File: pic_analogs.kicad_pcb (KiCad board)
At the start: 2 copper layers, 99.1 x 98.4 mm, 226 parts, among them J1 VFWD, J10 USB_B_Mini, J11 term_, J12 term_, J13 term_, J14 term_, J15 term_, J16 term_, J17 term_, J18 term_, J19 term_, J2 IN_RF, J20 term_, J21 term_, J22 term_, J23 term_, J24 term_, J25 term_, J26 term_, J27 term_, J28 term_, J29 term_, J3 OUT_RF, J30 term_, J31 term_, J32 ICD, J33 Micro_SD_Card, J34 Raspberry_Pi_zero_2w, J35 USB_A, J36 OledSpiST1306, J37 OledSpiST7789, J4 VREV, J42 OledSpiST1306, J43 tp_ft232_, J44 tp_ft232_, J45 tp_ft232_, J46 tp_ft232_, J47 tp_ft232_, J48 tp_ft232_, J49 tp_ft232_, J5 pickit, J50 tp_ft232_, J51 tp_ft232_, J52 USB_B_Mini, J53 F32R-1A7H1-11024, J54 tp_epaper, J56 tp_epaper, J57 tp_epaper, J58 tp_epaper, J59 tp_epaper, J6 oled128x64, J7 oled128x64, Q1 PMOS, SW1 mclr, SW2 rb4, SW3 rb5, SW4 mclr, SW5 ra5, SW6 ra4, SW7 ra5, U2 LM1117DT-3.3, U3 PIC18F4550-IPT, U5 MRF24J40MA, U6 FT232BM, U7 LM1117DT-3.3, U8 25LCxxx, Y1 Crystal_GND24_Small, Y2 6Mhz

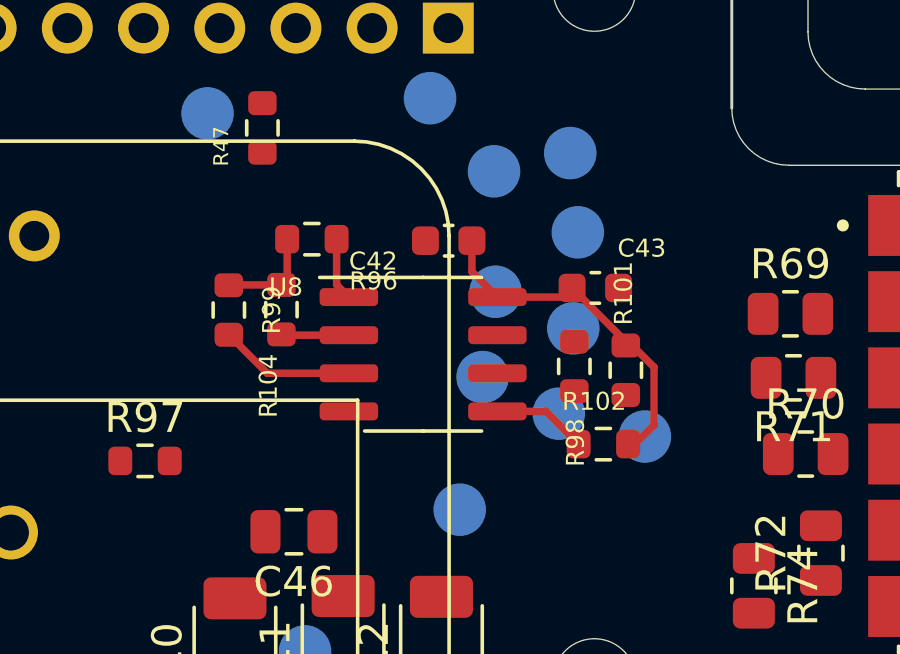
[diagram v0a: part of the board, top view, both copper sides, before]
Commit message: Update
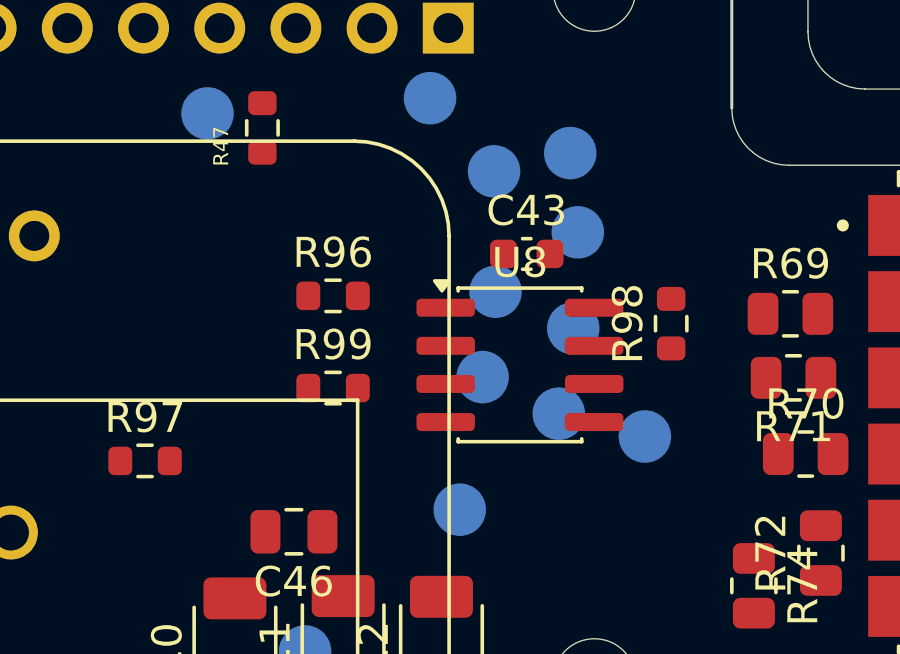
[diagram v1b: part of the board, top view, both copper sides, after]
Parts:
- removed C42: 100n, Capacitor_SMD:C_0603_1608Metric
- removed R101: 10K, Resistor_SMD:R_0603_1608Metric
- removed R102, R104: 2k2, Resistor_SMD:R_0603_1608Metric
- moved R99 4.34 mm to (175.3, 147.1), turned to 0 degrees
- moved R98 3.53 mm to (186.6, 145.0), turned to 90 degrees
- moved U8 3.25 mm to (181.5, 146.4)
- moved C43 2.55 mm to (181.8, 142.7)
- moved R96 2.02 mm to (175.3, 144.1)
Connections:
- U8 pad 2: MISO -> /magnetics/mcu_pic/rpi/mrf24j40/MISO_mrf24j40
- U8 pad 5: MOSI -> /magnetics/mcu_pic/rpi/mrf24j40/MOSI_mrf24j40
- U8 pad 6: SCLK -> /magnetics/mcu_pic/rpi/mrf24j40/SCLK_mrf24j40
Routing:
- net +3V3: track 15.2 -> 0.00 mm
- net Net-(U8-~{WP}): track 4.53 -> 0.00 mm
- net MOSI: track 3.16 -> 0.00 mm
- net MISO: track 2.26 -> 0.00 mm
- net CE1: track 2.10 -> 0.00 mm
